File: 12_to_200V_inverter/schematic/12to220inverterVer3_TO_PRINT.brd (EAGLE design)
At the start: 150 x 100 mm, 245 parts, among them IC1 UC3842, IC10 TL494, IC2 PC817, IC3 LM358SOIC8, IC4 TL431, IC5 LM317, IC6 74HC595, IC7 74HC595, IC8 ATTINY45, IC9 TL431, J2 0, J3 0, T1 AO4407AL, T10 16N60, T11 BC847, T12 BC847, T13 BSS84, T15 BC847, T16 BSS84, T17 BC847, T18 BC847, T19 BSS84, T2 IRF830, T20 BSS84, T21 BC847, T22 BC847, T23 BSS84, T24 BC847, T3 IRF830, T4 BC847, T5 BC857, T6 BC857, T7 IRFZ24N, T8 IRFZ24N, T9 BC857, X1 BAT+, X2 LAMP1, X3 LAMP1, X4 BAT-, X5 220VAC, X6 LAMP1_SWITCH, X7 LAMP1_SWITCH, X8 MCU_PROGRAMMING

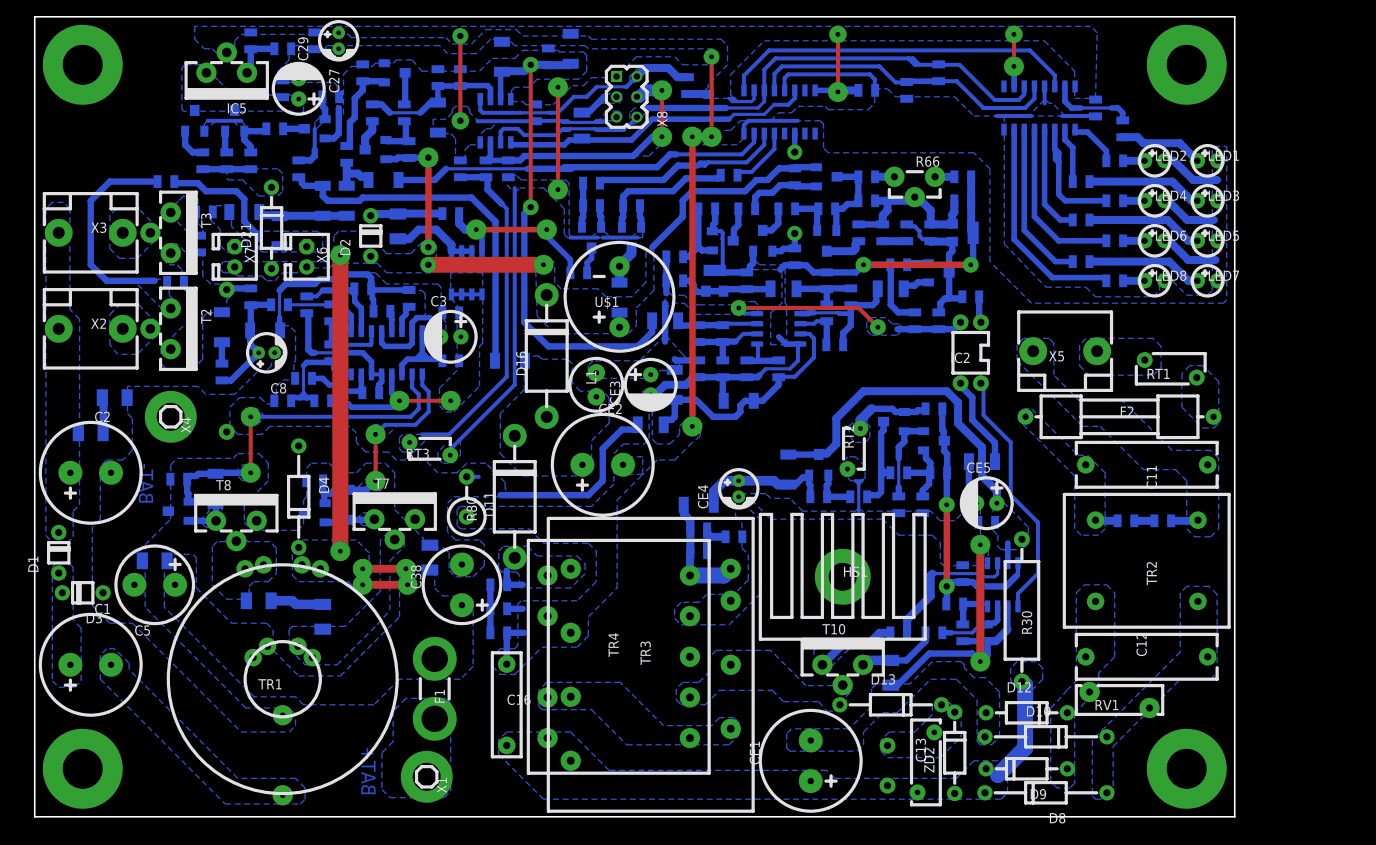
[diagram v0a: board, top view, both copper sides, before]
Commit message: 12 to 200V inverter. New board with ETD transformers. Finally routed.
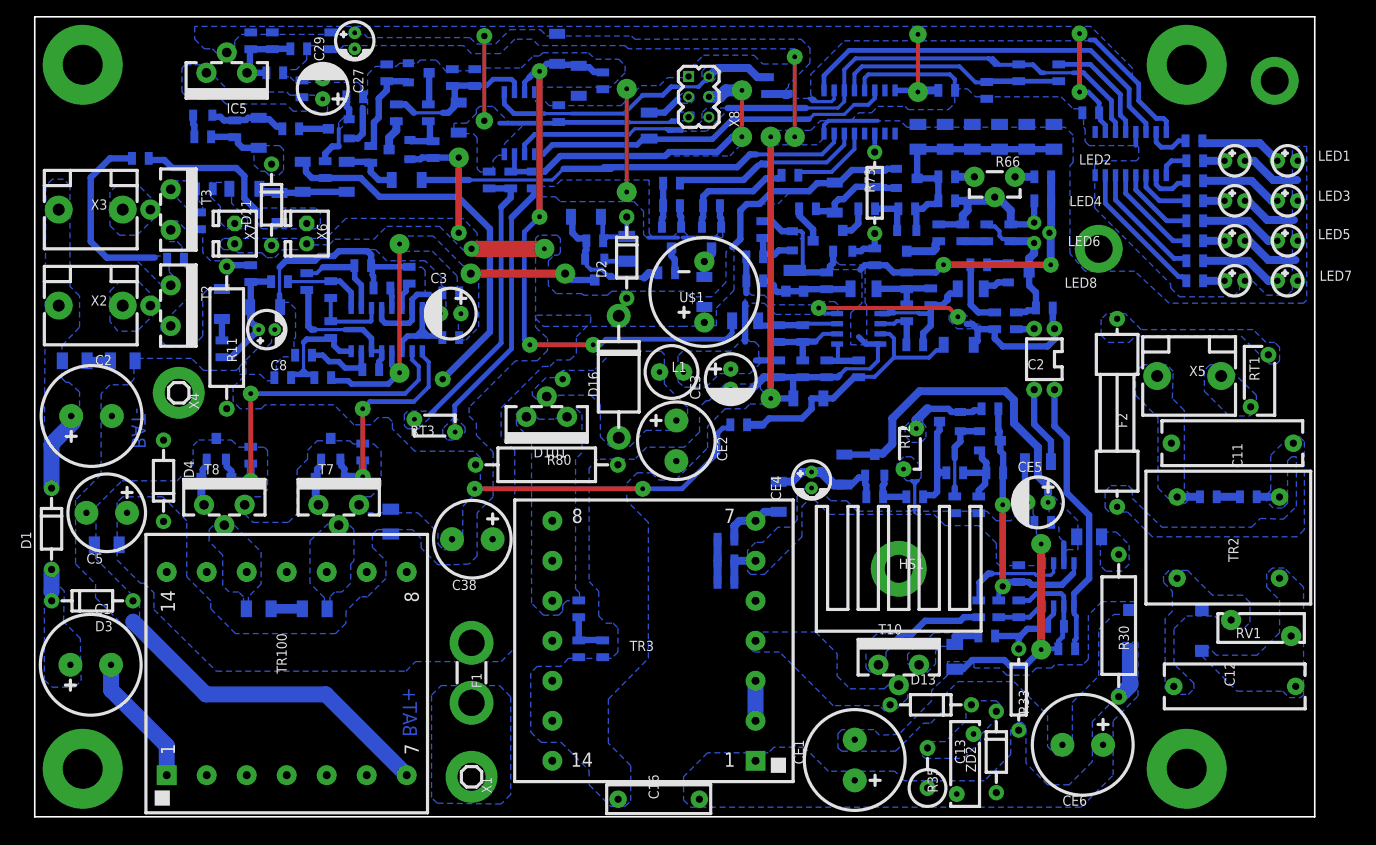
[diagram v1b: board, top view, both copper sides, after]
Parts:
- removed D10, D8: 1N4007, __MyCommonLib1:DO-41_15MM
- removed D11: SR3A0, __MyCommonLib1:DO-27_15MM
- removed D12, D9: 1N4007, __MyCommonLib1:DO-41_10MM
- removed T1: AO4407AL, __MyCommonLib1:SOIC8
- removed T20: BSS84, __MyCommonLib1:SOT23_SMALL_PADS
- removed TR1: 12_to_200_trans, __MyCommonLib1:RING_TRANSF_30X9_3WINGS
- removed TR4: Self made transformer. From TR8 sat reciever., __MyCommonLib1:TRANS_29.5X23_1234567_910
- added C40: 10nF*, __MyCommonLib1:RSMD_0805
- added CE6: 22uF x 400V, __MyCommonLib1:CE_13MM
- added D101: MBR20100CT, __MyCommonLib1:TO-220(VER2)_BIG_PADS
- added J100: 0, __MyCommonLib1:RSMD_1206
- added J101: 0, __MyCommonLib1:RSMD_0805
- added R33: 750K, __MyCommonLib1:R0207
- added R34, R36, R37, R38, R51, R56: 2K0, __MyCommonLib1:RSMD_1206
- added R69: *, __MyCommonLib1:RSMD_0805
- added T14: AO3401, __MyCommonLib1:SOT23_SMALL_PADS
- added TR100: 12_to_200_trans, __MyCommonLib1:ETD29_HOR
- added U100: DF06S, rectifier:DFS
- added ZD3, ZD4, ZD5: 5V6, __MyCommonLib1:SOD-80
- C19: value 1n0 x 16V* -> 10nF x 50V
- C23: value 10nF -> 47nF
- CE2: device __MyCommonLib1:CE_13MM -> __MyCommonLib1:CE_10MM
- CE5: value 22uFx50V -> 100uFx50V
- D1, D2, D3: device __MyCommonLib1:DO-41_5MM -> __MyCommonLib1:DO-41_10MM
- D13, D4: device __MyCommonLib1:DO-41_12.5MM -> __MyCommonLib1:DO-41_10MM
- D23: device __MyCommonLib1:SOD-80 -> __MyCommonLib1:DO-35_15MM
- IC3: value LM358SOIC8 -> LM358
- IC4: device __MyCommonLib1:SOT23 -> __MyCommonLib1:TO-92A(PINS_SWAPED)
- IC8: device __MyCommonLib1:SOIC8(0.15'') -> __MyCommonLib1:PSOP8(0.208'')
- LED1: value RED -> VOLT_GREEN2
- LED2: value GREEN -> CURR_RED
- LED3: value YELLOW -> VOLT_GREEN1
- LED4: value YELLOW -> CURR_YELLOW
- LED5: value YELLOW -> VOLT_YELLOW
- LED6: value YELLOW -> CURR_GREEN1
- LED7: value GREEN -> VOLT_RED
- LED8: value RED -> CURR_GREEN2
- R35: value 33K -> 33K* 2W
- R46: value 3K9* -> 9K1*
- R53: value 3K9* -> 330R
- R57: value 3R9 -> 2R4
- R65: value 1M0 -> 27K
- R76: device __MyCommonLib1:RSMD_1206_BIG_GAP -> __MyCommonLib1:RSMD_0805
- R80: device __MyCommonLib1:R_1.0W_VERTICAL -> __MyCommonLib1:R_1.0W
- R84: value 20R -> 10R
- R86: value 20R -> *
- T13: value BSS84 -> AO3401
- TR3: value Self made transformer. From TR8 sat reciever. -> ETD29_Transf; device __MyCommonLib1:TRANS_37X26_3578_11_13_15_17 -> __MyCommonLib1:ETD29_HOR
- moved D19 35.9 mm to (115.5, 59.0), turned to 0 degrees
- moved D2 32.1 mm to (74.0, 69.9)
- moved R1 28.7 mm to (74.0, 71.0)
- moved C16 22.4 mm to (78.0, 2.20), turned to 90 degrees
- moved RV1 19.9 mm to (153.3, 23.6)
- moved R4 18.3 mm to (70.0, 72.0), turned to 180 degrees
- moved D4 17.0 mm to (16.1, 42.0)
- moved X5 15.8 mm to (144.3, 55.1), turned to 0 degrees
- moved R101 14.2 mm to (145.0, 79.5)
- moved R103 14.2 mm to (145.0, 74.5)
- moved R105 14.2 mm to (145.0, 69.5)
- moved R61 13.3 mm to (126.2, 63.6), turned to 0 degrees
- moved R42 13.2 mm to (71.0, 21.0), turned to 270 degrees
- moved IC7 12.7 mm to (137.0, 82.9)
- moved R86 12.5 mm to (30.0, 93.0), turned to 0 degrees
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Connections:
- removed net N$125: R62.PAD_1, R63.PAD_1, R64.PAD_1, T13.3, T16.2
- new net N$13: IC2.2, R59.PAD_1
- new net N$63: R34.PAD_1, R36.PAD_1, R37.PAD_1, R38.PAD_1, R51.PAD_1, R56.PAD_1, R62.PAD_1, R63.PAD_1, R64.PAD_1, T13.3, T16.2
- net +12V_BAT: now also TR100.14, TR100.8, ZD3.CATHODE; no longer TR1.PRI_A_END1, TR1.PRI_A_END2, TR1.PRI_B_START1, TR1.PRI_B_START2
- net +12V_CONVERTER: now also T14.3; no longer T1.5, T1.6, T1.7, T1.8
- net +5V: now also R69.PAD_1
- net -VBAT: now also TR100.7; no longer TR1.SEC_START
- net CHARGER_POWER: now also D101.2, D23.A; no longer D11.CATHODE, D23.ANODE
- net GND: now also IC4.2, R34.PAD_0, R36.PAD_0, R37.PAD_0, R38.PAD_0, R51.PAD_0, R56.PAD_0, R86.PAD_0, TR3.12; no longer IC4.3, TR4.7
- net LED_LATCH: now also J101.PAD_0; no longer IC7.12
- net N$104: now also IC7.12, J101.PAD_1; no longer R86.PAD_1, T20.2
- net N$109: now also T14.2; no longer T1.1, T1.2, T1.3
- net N$14: now also T14.1, ZD4.CATHODE; no longer T1.4
- net N$15: now also ZD5.CATHODE; no longer R86.PAD_0
- net N$22: now also F2.PAD1; no longer X5.2
- net N$24: now also TR100.10; no longer TR1.PRI_A_START1, TR1.PRI_A_START2
- net N$25: now also TR100.12; no longer TR1.PRI_B_END1, TR1.PRI_B_END2
- net N$27: now also X5.1; no longer F2.PAD_0
- net N$28: now also U100.AC2; no longer D12.CATHODE, D9.ANODE
- net N$29: now also U100.AC1; no longer D10.CATHODE, D8.ANODE
- net N$32: now also CE6.PLUS, R33.PAD1, TR3.1, U100.+; no longer D8.CATHODE, D9.CATHODE, TR3.17, TR4.10
- net N$34: now also TR3.2; no longer TR3.15, TR4.1, TR4.9
- net N$35: now also TR3.4; no longer TR3.5, TR4.2
- net N$38: now also J100.PAD_0; no longer R30.PAD_0
- net N$40: now also RT1.PAD_0, X5.2; no longer IC2.1, R59.PAD_1
- net N$43: now also R33.PAD_0
- net N$48: now also C15.PAD_1, TR3.7; no longer R47.PAD_0, R48.PAD_0, TR3.8, TR4.5
- net N$49: now also C15.PAD_0, R47.PAD_0, R48.PAD_0; no longer C15.PAD_1, R47.PAD_1, R48.PAD_1
- net N$50: now also C40.PAD_0, CE6.MINUS, R47.PAD_1, R48.PAD_1, TR3.6, U100.-; no longer C15.PAD_0, D10.ANODE, D12.ANODE, TR3.7, TR4.4
- net N$55: now also C40.PAD_1
- net N$58: now also D101.1, D101.3, TR3.10, TR3.9; no longer D11.ANODE, TR3.11, TR4.6
- net N$59: now also ZD5.ANODE; no longer T20.1
- net N$61: now also F2.PAD_0, RT1.PAD1; no longer F2.PAD1, RT1.PAD_0
- net N$62: now also IC4.3; no longer IC4.1
- net N$68: now also IC4.1; no longer IC4.2
- net N$70: now also J100.PAD_1, R30.PAD_0; no longer RT1.PAD1, X5.1
- net N$74: now also R69.PAD_0, R86.PAD_1
- net N$8: now also TR100.1; no longer TR1.SEC_END
- net N$9: now also ZD4.ANODE
- net N$91: no longer T20.3
- net N$93: now also D23.C; no longer D23.CATHODE
- net N$95: now also ZD3.ANODE
- net N$98: now also IC2.1; no longer IC2.2
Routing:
- net -VBAT: track 61.9 -> 115.9 mm, vias 0 -> 2
- net +12V_BAT: track 105.1 -> 51.7 mm, vias 10 -> 4
- net N$63: track 0.00 -> 32.6 mm
- net +5V: track 56.8 -> 86.1 mm
- net +12V_CONVERTER: track 23.2 -> 44.6 mm, vias 2 -> 4
- net GND: track 269.2 -> 249.6 mm, vias 8 -> 9
- net N$8: track 0.00 -> 16.7 mm
- net N$125: track 11.7 -> 0.00 mm
- net N$104: track 2.73 -> 14.2 mm
- net CHARGE_CURR_ADC: track 64.5 -> 75.1 mm, vias 2 -> 4
- net N$98: track 41.6 -> 52.0 mm
- net LED_LATCH: track 39.2 -> 28.9 mm
- net N$82: track 27.4 -> 17.7 mm
- net +200VDC_OUT: track 0.00 -> 9.34 mm
- net N$78: track 16.4 -> 7.25 mm
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- added copper zone on layer 16, net N$37
- added copper zone on layer 16, net N$40
- removed copper zone on layer 16, net CONV_PWM1
- removed copper zone on layer 16, net CONV_PWM2
- removed copper zone on layer 16, net N$19
- removed copper zone on layer 16, net N$21
- removed copper zone on layer 16, net N$34
- removed copper zone on layer 16, net N$59
- removed copper zone on layer 16, net N$8
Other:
- board size 150 x 100 mm -> 160 x 100 mm
